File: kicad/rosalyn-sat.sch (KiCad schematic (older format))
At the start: 18 parts, among them J2 Serial, U1 STM32F030F4Px, U2 E22-EBYTE, U3 XC6206P330MR

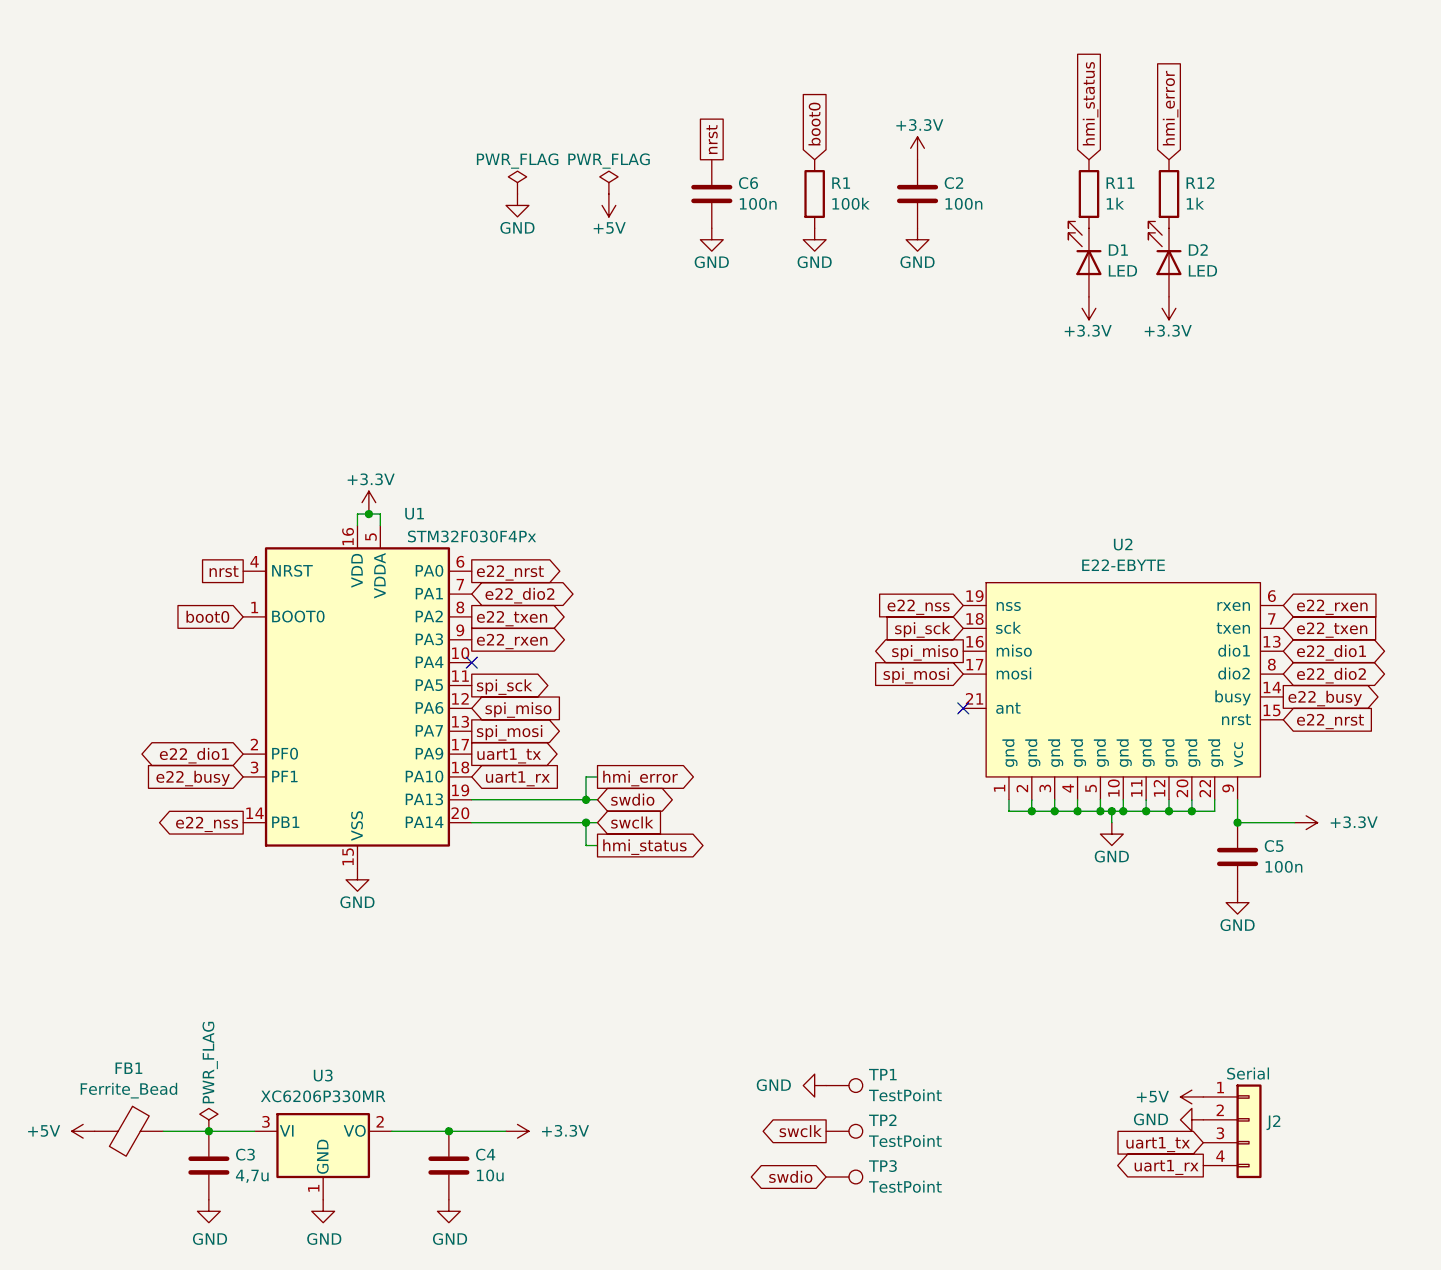
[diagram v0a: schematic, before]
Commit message: Tage (#2)
* rosalyn-sat_v1.0

* added nvdata driver

* removed kicad bak files

* removed stm32__ folder
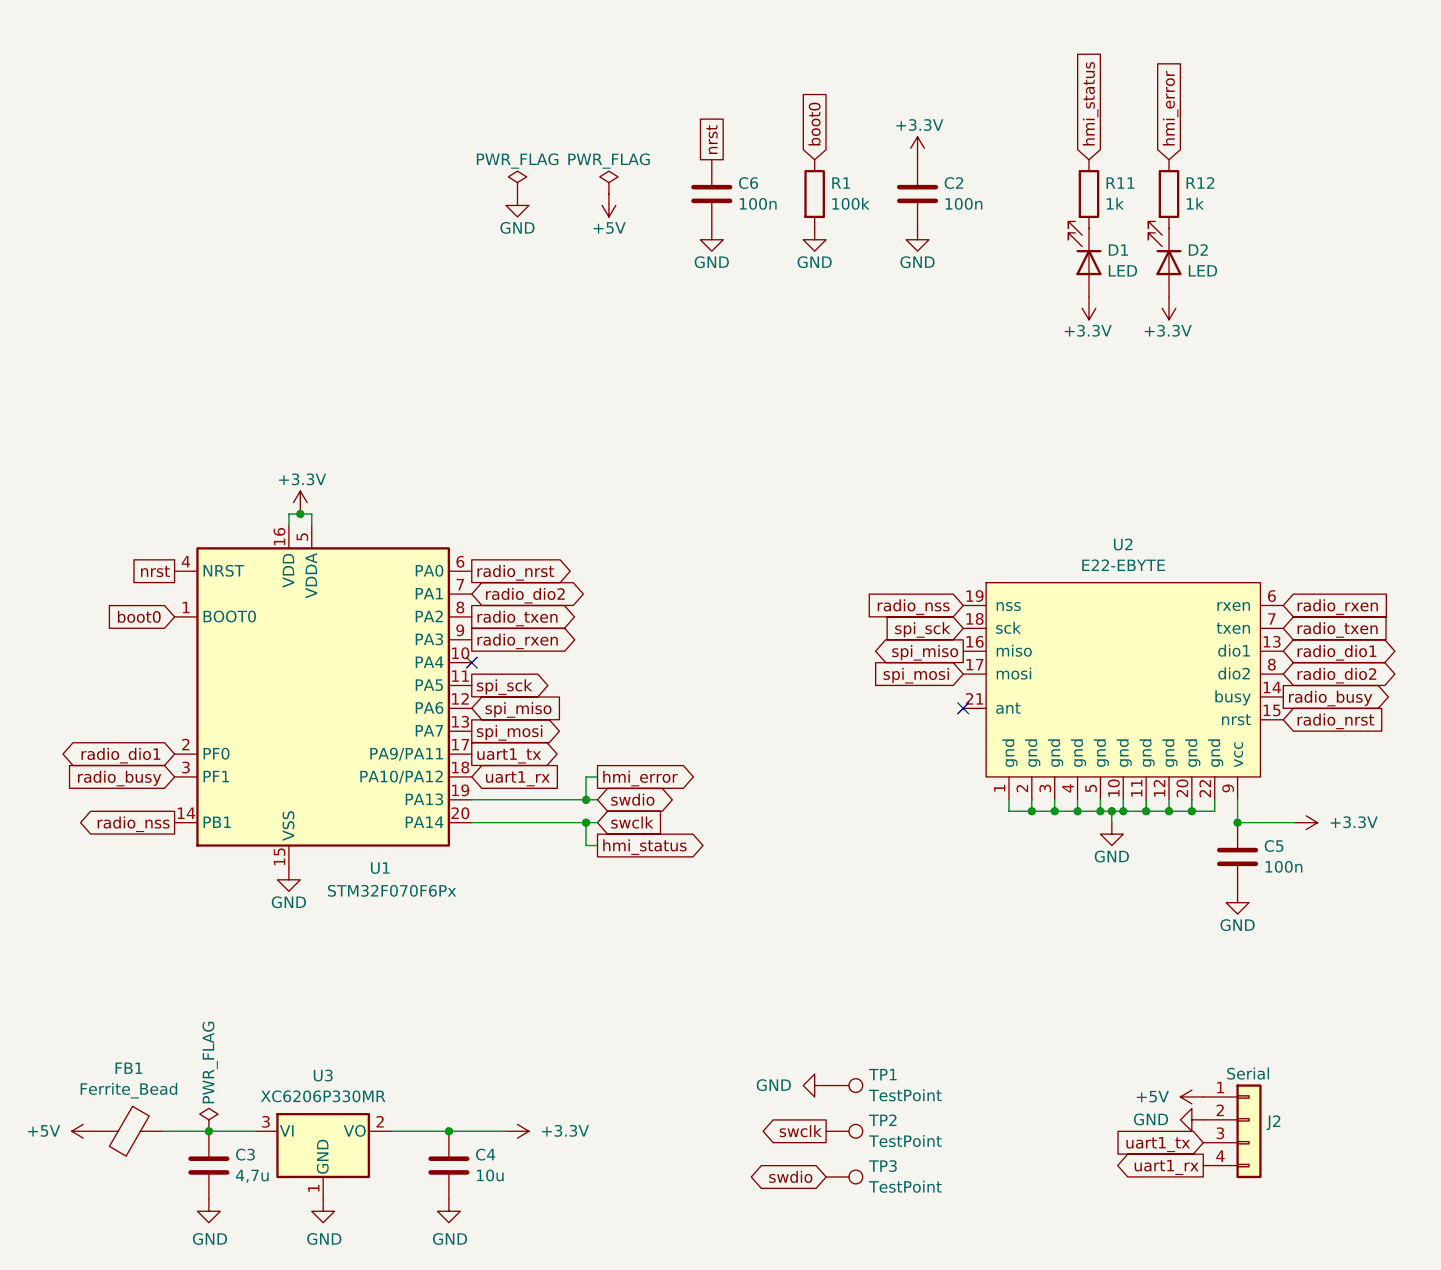
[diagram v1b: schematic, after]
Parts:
- removed U1: STM32F030F4Px, Package_SO:TSSOP-20_4.4x6.5mm_P0.65mm, symbol MCU_ST_STM32F0:STM32F030F4Px
- added U1: STM32F070F6Px, Package_SO:TSSOP-20_4.4x6.5mm_P0.65mm, symbol MCU_ST_STM32F0:STM32F070F6Px
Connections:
- net +3V3: now also U1.16 (VDD), U1.5 (VDDA)
- net GND: now also U1.15 (VSS)
- net boot0: now also U1.1 (BOOT0)
- net hmi_error: now also U1.19 (PA13)
- net hmi_status: now also U1.20 (PA14)
- net nrst: now also U1.4 (NRST)
- net spi_miso: now also U1.12 (PA6)
- net spi_mosi: now also U1.13 (PA7)
- net spi_sck: now also U1.11 (PA5)
- net uart1_rx: now also U1.18 (PA10/PA12)
- net uart1_tx: now also U1.17 (PA9/PA11)
- net e22_busy renamed radio_busy
- net radio_busy: now also U1.3 (PF1)
- net e22_dio1 renamed radio_dio1
- net radio_dio1: now also U1.2 (PF0)
- net e22_dio2 renamed radio_dio2
- net radio_dio2: now also U1.7 (PA1)
- net e22_nrst renamed radio_nrst
- net radio_nrst: now also U1.6 (PA0)
- net e22_nss renamed radio_nss
- net radio_nss: now also U1.14 (PB1)
- net e22_rxen renamed radio_rxen
- net radio_rxen: now also U1.9 (PA3)
- net e22_txen renamed radio_txen
- net radio_txen: now also U1.8 (PA2)
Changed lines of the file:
@@
 $EndComp
 Text GLabel 8050 3100 2    50   Input ~ 0
-e22_rxen
+radio_rxen
 Text GLabel 8050 3300 2    50   BiDi ~ 0
-e22_dio1
+radio_dio1
 Text GLabel 8050 3500 2    50   Output ~ 0
-e22_busy
+radio_busy
 Text GLabel 8050 3600 2    50   Input ~ 0
-e22_nrst
+radio_nrst
 Text GLabel 6650 3100 0    50   Input ~ 0
-e22_nss
+radio_nss
 Text GLabel 6650 3200 0    50   Input ~ 0
 spi_sck
@@
 Text GLabel 5550 1150 1    50   UnSpc ~ 0
 nrst
-$Comp
-L MCU_ST_STM32F0:STM32F030F4Px U1
-U 1 1 5FB02EA0
-P 4000 3450
-F 0 "U1" H 4250 4200 50  0000 C CNN
-F 1 "STM32F030F4Px" H 4500 4100 50  0000 C CNN
-F 2 "Package_SO:TSSOP-20_4.4x6.5mm_P0.65mm" H 3600 2750 50  0001 R CNN
-F 3 "http://www.st.com/st-web-ui/static/active/en/resource/technical/document/datasheet/DM00088500.pdf" H 4000 3450 50  0001 C CNN
-	1    4000 3450
-	1    0    0    -1
-$EndComp
 Text GLabel 4500 3750 2    50   Output ~ 0
 uart1_tx
@@
 Text GLabel 5050 3850 2    50   Output ~ 0
 hmi_error
-Text GLabel 3500 4050 0    50   Output ~ 0
-e22_nss
+Text GLabel 3200 4050 0    50   Output ~ 0
+radio_nss
 Text GLabel 4500 2950 2    50   Output ~ 0
-e22_nrst
-Text GLabel 3500 2950 0    50   UnSpc ~ 0
+radio_nrst
+Text GLabel 3200 2950 0    50   UnSpc ~ 0
 nrst
 $Comp
 L power:+3.3V #PWR09
 U 1 1 5FB2A297
-P 4050 2700
-F 0 "#PWR09" H 4050 2550 50  0001 C CNN
-F 1 "+3.3V" H 3950 2850 50  0000 L CNN
-F 2 "" H 4050 2700 50  0001 C CNN
-F 3 "" H 4050 2700 50  0001 C CNN
-	1    4050 2700
-	1    0    0    -1
-$EndComp
-Wire Wire Line
-	4100 2750 4100 2700
-Wire Wire Line
-	4100 2700 4050 2700
-Wire Wire Line
-	4000 2750 4000 2700
-Wire Wire Line
-	4000 2700 4050 2700
-Connection ~ 4050 2700
-Text GLabel 3500 3150 0    50   Input ~ 0
+P 3750 2700
+F 0 "#PWR09" H 3750 2550 50  0001 C CNN
+F 1 "+3.3V" H 3650 2850 50  0000 L CNN
+F 2 "" H 3750 2700 50  0001 C CNN
+F 3 "" H 3750 2700 50  0001 C CNN
+	1    3750 2700
+	1    0    0    -1
+$EndComp
+Text GLabel 3200 3150 0    50   Input ~ 0
 boot0
 Text GLabel 6000 1150 1    50   Input ~ 0
@@
 L power:GND #PWR012
 U 1 1 5FB65C99
-P 4000 4250
-F 0 "#PWR012" H 4000 4000 50  0001 C CNN
-F 1 "GND" H 4000 4100 50  0000 C CNN
-F 2 "" H 4000 4250 50  0001 C CNN
-F 3 "" H 4000 4250 50  0001 C CNN
-	1    4000 4250
+P 3700 4250
+F 0 "#PWR012" H 3700 4000 50  0001 C CNN
+F 1 "GND" H 3700 4100 50  0000 C CNN
+F 2 "" H 3700 4250 50  0001 C CNN
+F 3 "" H 3700 4250 50  0001 C CNN
+	1    3700 4250
 	1    0    0    -1
 $EndComp
@@
 	0    1    1    0
 $EndComp
-Text GLabel 3500 3850 0    50   Input ~ 0
-e22_busy
-Text GLabel 3500 3750 0    50   BiDi ~ 0
-e22_dio1
+Text GLabel 3200 3850 0    50   Input ~ 0
+radio_busy
+Text GLabel 3200 3750 0    50   BiDi ~ 0
+radio_dio1
 Text GLabel 4500 3250 2    50   Output ~ 0
-e22_rxen
+radio_rxen
 Text GLabel 8050 3200 2    50   Input ~ 0
-e22_txen
+radio_txen
 Text GLabel 8050 3400 2    50   BiDi ~ 0
-e22_dio2
+radio_dio2
 Text GLabel 4500 3050 2    50   BiDi ~ 0
-e22_dio2
+radio_dio2
 Text GLabel 4500 3150 2    50   Output ~ 0
-e22_txen
+radio_txen
 $Comp
 L Device:Ferrite_Bead FB1
@@
 	1    0    0    -1
 $EndComp
+Wire Wire Line
+	3700 2750 3700 2700
+Wire Wire Line
+	3800 2700 3800 2750
+Wire Wire Line
+	3700 2700 3750 2700
+Connection ~ 3750 2700
+Wire Wire Line
+	3750 2700 3800 2700
+$Comp
+L MCU_ST_STM32F0:STM32F070F6Px U1
+U 1 1 5FC13811
+P 3900 3450
+F 0 "U1" H 4100 2650 50  0000 C CNN
+F 1 "STM32F070F6Px" H 4150 2550 50  0000 C CNN
+F 2 "Package_SO:TSSOP-20_4.4x6.5mm_P0.65mm" H 3300 2750 50  0001 R CNN
+F 3 "http://www.st.com/st-web-ui/static/active/en/resource/technical/document/datasheet/DM00141386.pdf" H 3900 3450 50  0001 C CNN
+	1    3900 3450
+	1    0    0    -1
+$EndComp
